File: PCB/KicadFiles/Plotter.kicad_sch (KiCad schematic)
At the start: 2 parts, among them U1 TMC2209-V1.2_Bigtreetech, U2 ESP32-WROOM-32

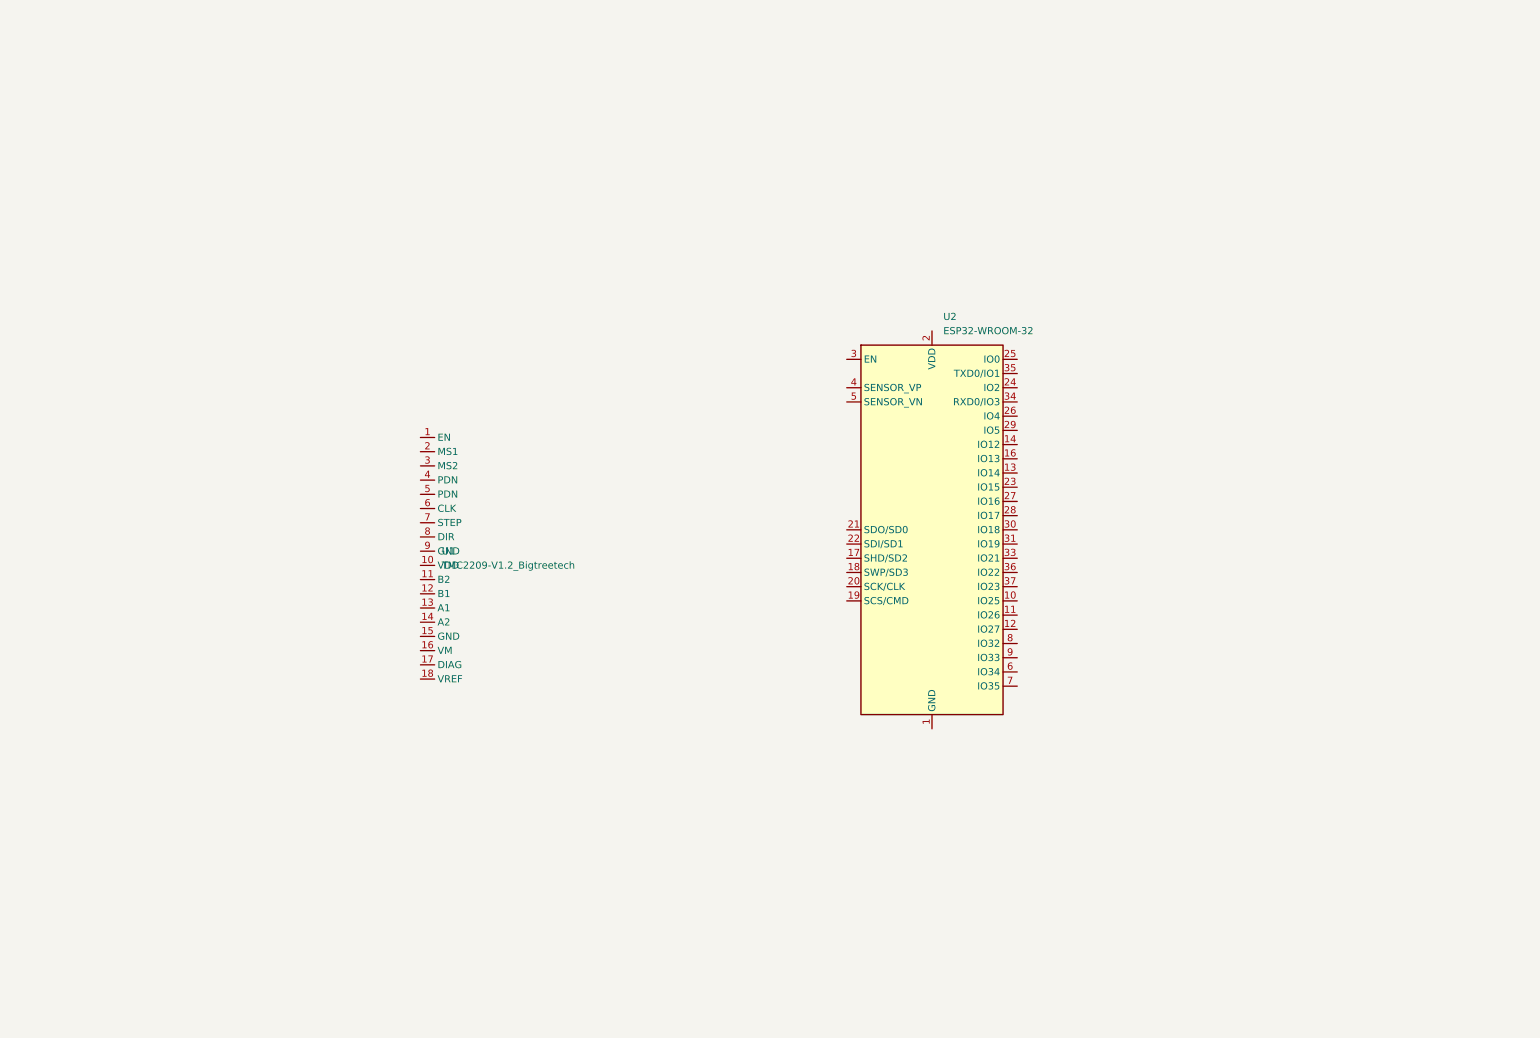
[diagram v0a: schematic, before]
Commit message: schematic half way done
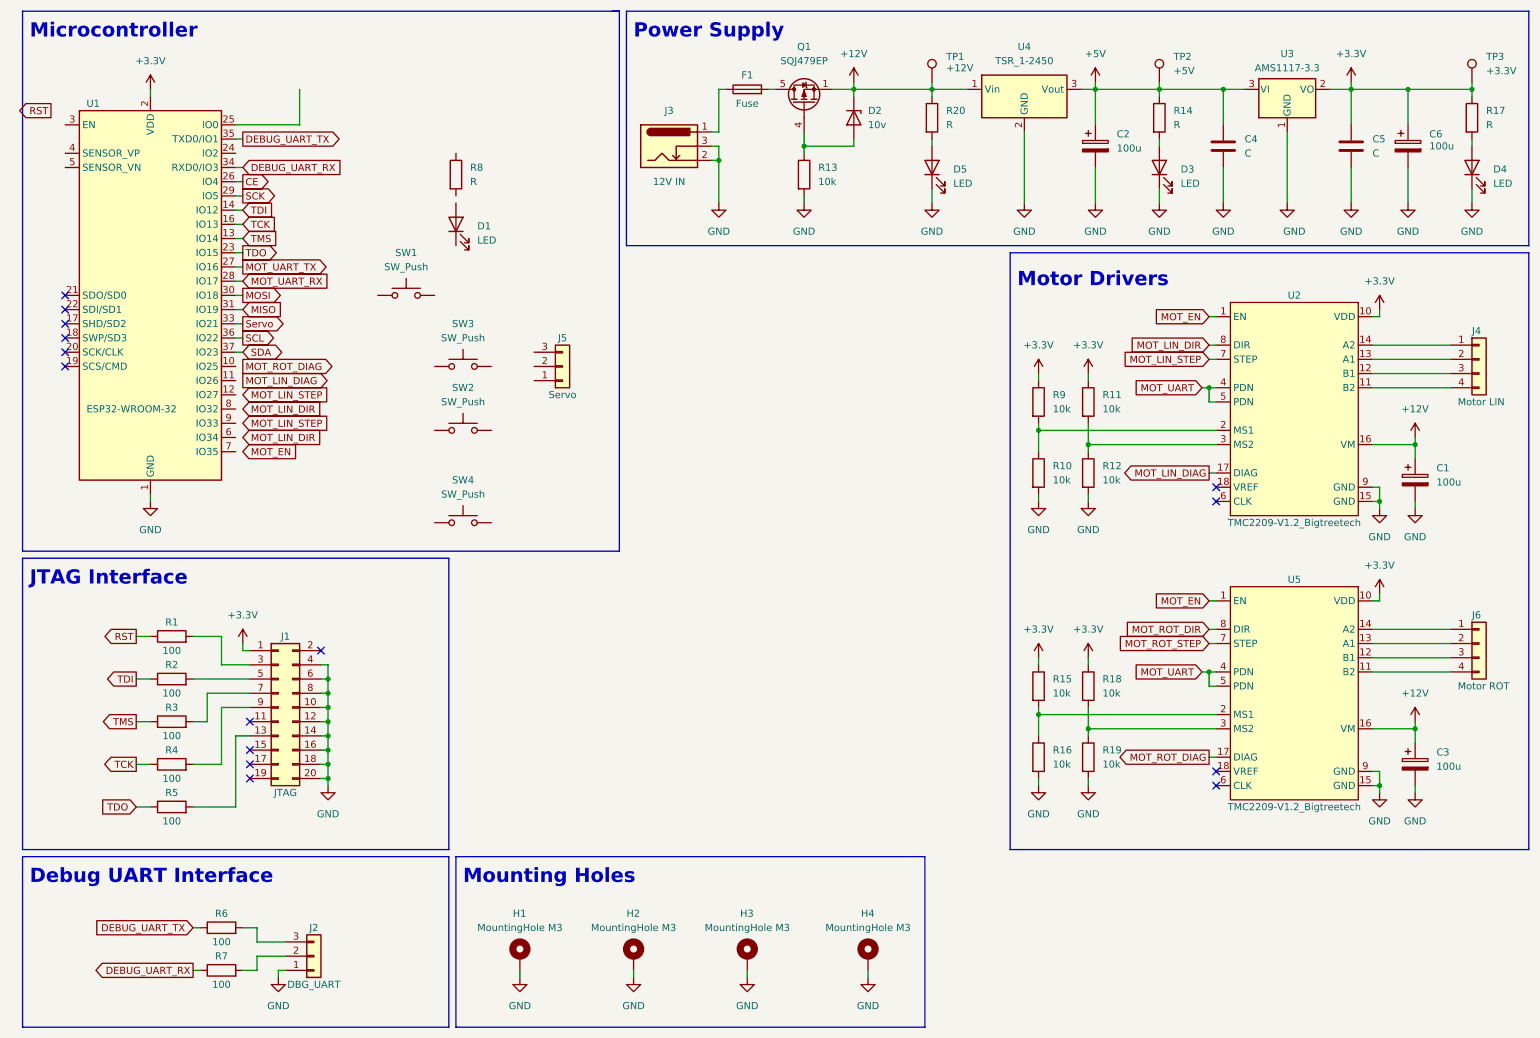
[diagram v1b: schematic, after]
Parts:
- removed U1: TMC2209-V1.2_Bigtreetech, Footprints:TMC2209-V1.2 Bigtreetech, symbol Symbols:TMC2209-V1.2_Bigtreetech
- added C1, C2, C3, C6: 100u, Capacitor_SMD:CP_Elec_6.3x7.7, symbol Device:C_Polarized
- added C4, C5: C, Capacitor_SMD:C_0603_1608Metric, symbol Device:C
- added D1, D3, D4, D5: LED, LED_SMD:LED_0603_1608Metric, symbol Device:LED
- added D2: 10v, Package_TO_SOT_SMD:SOT-23, symbol Diode:BZX84Cxx
- added F1: Fuse, Fuse:Fuseholder_Cylinder-5x20mm_Schurter_0031_8201_Horizontal_Open, symbol Device:Fuse
- added H1, H2, H3, H4: MountingHole M3, MountingHole:MountingHole_3.2mm_M3_Pad_Via, symbol Mechanical:MountingHole_Pad
- added J1: JTAG, Connector_IDC:IDC-Header_2x10_P2.54mm_Vertical, symbol Connector_Generic:Conn_02x10_Odd_Even
- added J2: DBG_UART, Connector_JST:JST_XH_B3B-XH-A_1x03_P2.50mm_Vertical, symbol Connector_Generic:Conn_01x03
- added J3: 12V IN, Connector_BarrelJack:BarrelJack_CLIFF_FC681465S_SMT_Horizontal, symbol Connector:Barrel_Jack_Switch
- added J4: Motor LIN, Connector_JST:JST_XH_B4B-XH-A_1x04_P2.50mm_Vertical, symbol Connector_Generic:Conn_01x04
- added J5: Servo, Connector_JST:JST_XH_B3B-XH-A_1x03_P2.50mm_Vertical, symbol Connector_Generic:Conn_01x03
- added J6: Motor ROT, Connector_JST:JST_XH_B4B-XH-A_1x04_P2.50mm_Vertical, symbol Connector_Generic:Conn_01x04
- added Q1: SQJ479EP, Package_TO_SOT_SMD:TDSON-8-1, symbol Transistor_FET:Si7141DP
- added R1, R2, R3, R4, R5, R6, R7: 100, Resistor_SMD:R_0603_1608Metric, symbol Device:R
- added R10, R11, R12, R13, R15, R16, R18, R19, R9: 10k, Resistor_SMD:R_0603_1608Metric, symbol Device:R
- added R14, R17, R20, R8: R, Resistor_SMD:R_0603_1608Metric, symbol Device:R
- added SW1, SW2, SW3, SW4: SW_Push, Button_Switch_THT:SW_PUSH_6mm_H5mm, symbol Switch:SW_Push
- added TP1: +12V, TestPoint:TestPoint_Loop_D2.54mm_Drill1.5mm_Beaded, symbol Connector:TestPoint
- added TP2: +5V, TestPoint:TestPoint_Loop_D2.54mm_Drill1.5mm_Beaded, symbol Connector:TestPoint
- added TP3: +3.3V, TestPoint:TestPoint_Loop_D2.54mm_Drill1.5mm_Beaded, symbol Connector:TestPoint
- added U2, U5: TMC2209-V1.2_Bigtreetech, Footprints:TMC2209-V1.2 Bigtreetech, symbol Symbols:TMC2209-V1.2_Bigtreetech
- added U3: AMS1117-3.3, Package_TO_SOT_SMD:SOT-223-3_TabPin2, symbol Regulator_Linear:AMS1117-3.3
- added U4: TSR_1-2450, Converter_DCDC:Converter_DCDC_TRACO_TSR-1_THT, symbol Regulator_Switching:TSR_1-2450
- renumbered U2 to U1
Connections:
- net GND: now reaches U1.1 (GND), U1.15 (GND), U1.38 (GND), U1.39 (GND)
- net GND: now also C1.2, C2.2, C3.2, C4.2, C5.2, C6.2, D3.1 (K), D4.1 (K), D5.1 (K), H1.1, H2.1, H3.1, H4.1, J1.10 (Pin_10), J1.12 (Pin_12), J1.14 (Pin_14), J1.16 (Pin_16), J1.18 (Pin_18), J1.20 (Pin_20), J1.4 (Pin_4), J1.6 (Pin_6), J1.8 (Pin_8), J2.1 (Pin_1), J3.2, J3.3, R10.2, R12.2, R13.2, R16.2, R19.2, U2.15 (GND), U2.9 (GND), U3.1 (GND), U4.2 (GND), U5.15 (GND), U5.9 (GND)
- net TMS: now reaches U1.13 (IO14)
- net TMS: now also R3.1
- net TDI: now reaches U1.14 (IO12)
- net TDI: now also R2.1
- net TCK: now reaches U1.16 (IO13)
- net TCK: now also R4.1
- net +3.3V: now reaches U1.2 (VDD)
- net +3.3V: now also C5.1, C6.1, J1.1 (Pin_1), R11.1, R15.1, R17.1, R18.1, R9.1, TP3.1, U2.10 (VDD), U3.2 (VO), U5.10 (VDD)
- net TDO: now reaches U1.23 (IO15)
- net TDO: now also R5.1
- net CE: now reaches U1.26 (IO4)
- net MOT_UART_TX: now reaches U1.27 (IO16)
- net MOT_UART_RX: now reaches U1.28 (IO17)
- net SCK: now reaches U1.29 (IO5)
- net MOSI: now reaches U1.30 (IO18)
- net MISO: now reaches U1.31 (IO19)
- net Servo: now reaches U1.33 (IO21)
- net DEBUG_UART_RX: now reaches U1.34 (RXD0/IO3)
- net DEBUG_UART_RX: now also R7.1
- net DEBUG_UART_TX: now reaches U1.35 (TXD0/IO1)
- net DEBUG_UART_TX: now also R6.1
- net SCL: now reaches U1.36 (IO22)
- net SDA: now reaches U1.37 (IO23)
- new net: R15.2, R16.1, U5.2 (MS1)
- new net: J1.7 (Pin_7), R3.2
- new net: R11.2, R12.1, U2.3 (MS2)
- new net: J6.4 (Pin_4), U5.11 (B2)
- new net: J6.3 (Pin_3), U5.12 (B1)
- new net: J6.2 (Pin_2), U5.13 (A1)
- new net: J6.1 (Pin_1), U5.14 (A2)
- new net: R18.2, R19.1, U5.3 (MS2)
- new net: J2.2 (Pin_2), R7.2
- new net: J2.3 (Pin_3), R6.2
- new net: F1.1, J3.1
- new net: D4.2 (A), R17.2
- new net: D2.1 (A), Q1.4 (G), R13.1
- new net: J4.1 (Pin_1), U2.14 (A2)
- new net: J4.2 (Pin_2), U2.13 (A1)
- new net: J4.3 (Pin_3), U2.12 (B1)
- new net: J4.4 (Pin_4), U2.11 (B2)
- new net: J1.13 (Pin_13), R5.2
- new net: J1.3 (Pin_3), R1.2
- new net: J1.5 (Pin_5), R2.2
- new net: J1.9 (Pin_9), R4.2
- new net: D3.2 (A), R14.2
- new net: R10.1, R9.2, U2.2 (MS1)
- new net: D5.2 (A), R20.2
- new net: F1.2, Q1.5 (D)
- new net +12V: C1.1, C3.1, D2.3 (K), Q1.1 (S), Q1.2 (S), Q1.3 (S), R20.1, TP1.1, U2.16 (VM), U4.1 (Vin), U5.16 (VM)
- new net +5V: C2.1, C4.1, R14.1, TP2.1, U3.3 (VI), U4.3 (Vout)
- new net MOT_EN: U2.1 (EN), U5.1 (EN)
- new net MOT_LIN_DIAG: U2.17 (DIAG)
- new net MOT_LIN_DIR: U2.8 (DIR)
- new net MOT_LIN_STEP: U2.7 (STEP)
- new net MOT_ROT_DIAG: U5.17 (DIAG)
- new net MOT_ROT_DIR: U5.8 (DIR)
- new net MOT_ROT_STEP: U5.7 (STEP)
- new net MOT_UART: U2.4 (PDN), U2.5 (PDN), U5.4 (PDN), U5.5 (PDN)
- new net RST: R1.1
- no-connect marks 0 -> 15
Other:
- note added: "Debug UART Interface"
- note added: "JTAG Interface"
- note added: "Microcontroller"
- note added: "Motor Drivers"
- note added: "Mounting Holes"
- note added: "Power Supply"
- company: (none) -> Lorenz Geisser
- title: (none) -> Plotter
- moved on the sheet: U1
